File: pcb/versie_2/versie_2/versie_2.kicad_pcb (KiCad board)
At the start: 2 copper layers, 100 x 63.5 mm, 7 parts, among them J2 Conn_01x04_Pin, J3 B4B-PH-SM4-TB__LF__SN_, U1 DFR0478

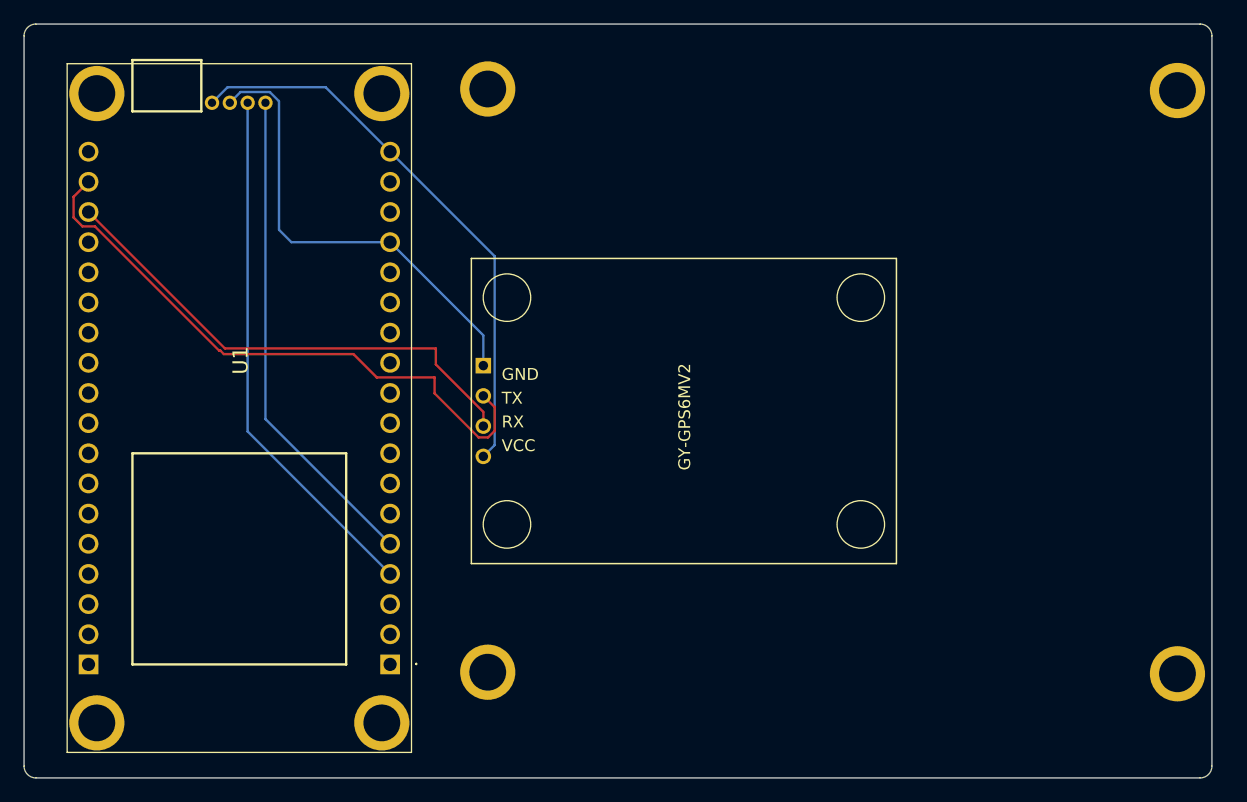
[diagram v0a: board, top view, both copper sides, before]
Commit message: pcb_update
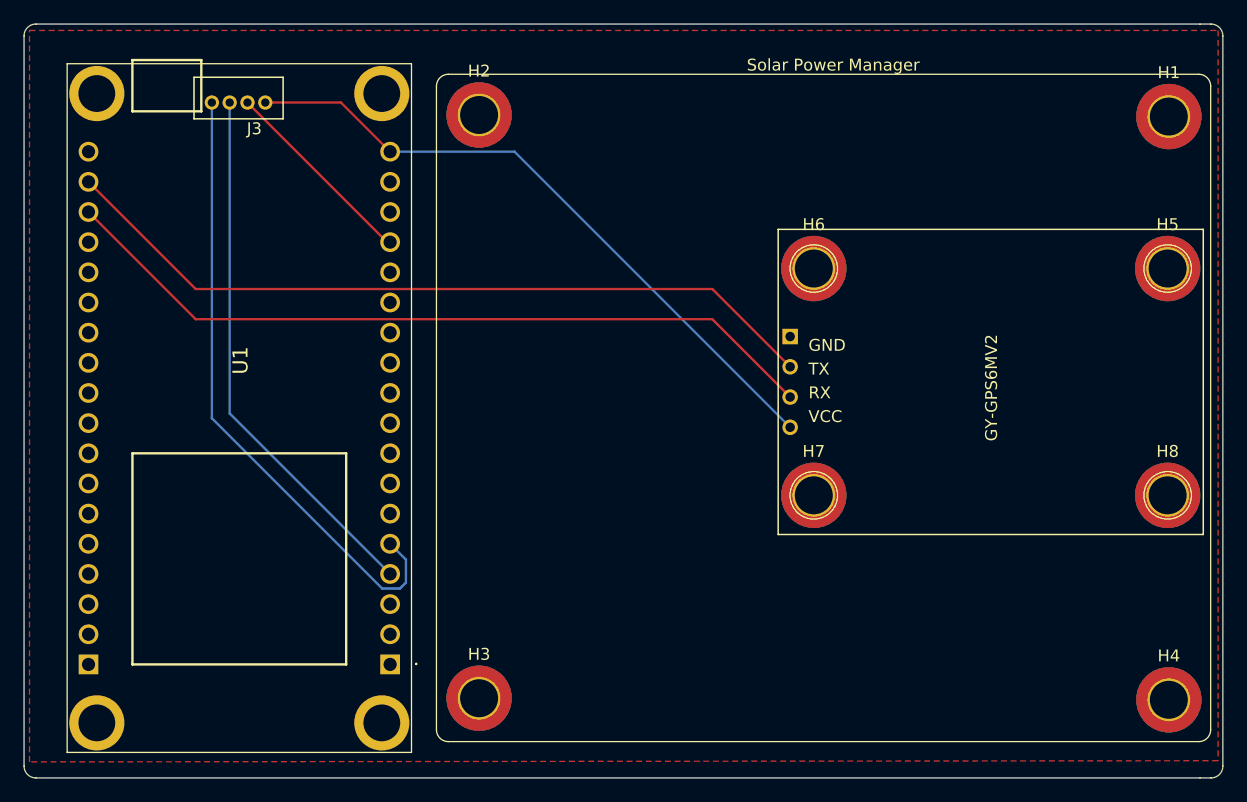
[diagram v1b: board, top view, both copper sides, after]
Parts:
- removed ? (x4): , 
- added H1: MountingHole_Pad, MountingHole:MountingHole_3.2mm_M3_ISO14580_Pad_TopBottom, F.Cu at (189.8, 71.8)
- added H2: MountingHole_Pad, MountingHole:MountingHole_3.2mm_M3_ISO14580_Pad_TopBottom, F.Cu at (131.7, 71.6)
- added H3: MountingHole_Pad, MountingHole:MountingHole_3.2mm_M3_ISO14580_Pad_TopBottom, F.Cu at (131.7, 120.7)
- added H4: MountingHole_Pad, MountingHole:MountingHole_3.2mm_M3_ISO14580_Pad_TopBottom, F.Cu at (189.8, 120.9)
- added H5: MountingHole_Pad, MountingHole:MountingHole_3.2mm_M3_ISO14580_Pad_TopBottom, F.Cu at (189.7, 84.5)
- added H6: MountingHole_Pad, MountingHole:MountingHole_3.2mm_M3_ISO14580_Pad_TopBottom, F.Cu at (159.8, 84.5)
- added H7: MountingHole_Pad, MountingHole:MountingHole_3.2mm_M3_ISO14580_Pad_TopBottom, F.Cu at (159.8, 103.7)
- added H8: MountingHole_Pad, MountingHole:MountingHole_3.2mm_M3_ISO14580_Pad_TopBottom, F.Cu at (189.7, 103.7)
- J3: moved to F.Cu
- moved J2 26.0 mm to (174.9, 94.1)
- moved J3 7.49 mm to (115.2, 71.9), turned to 180 degrees
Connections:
- U1 pad MH1: unconnected-(U1-PadMH1) -> GND
- U1 pad MH2: unconnected-(U1-PadMH2) -> GND
- U1 pad MH3: unconnected-(U1-PadMH3) -> GND
- U1 pad MH4: unconnected-(U1-PadMH4) -> GND
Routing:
- net RX: track 42.2 -> 65.5 mm
- net GND: track 39.6 -> 17.4 mm
- net TX: track 51.0 -> 65.5 mm
- net TX_1: track 41.7 -> 52.9 mm
- net vcc: track 47.5 -> 55.7 mm
- net RX_1: track 44.7 -> 45.3 mm
- added copper zone on F.Cu, net GND
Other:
- board size 100 x 63.5 mm -> 101 x 63.5 mm
- board text added: "Solar Power Manager"
